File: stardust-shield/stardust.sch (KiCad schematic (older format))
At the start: 56 parts, among them J1 BEXUS 28V, J2 Pololu J8557, J3 Pololu J8557, J4 Pololu J9251, J5 Pololu J9251 Servo, J6 DS3231M, J7 VMA430, J7'1 VMA430, SW1 SW_Push, SW2 SW_Push, U1 INA181, U2 INA181, U3 INA181, U4 INA181, U5 DS18B20, U6 DS18B20, U8 DHT22, U9 SSCDRNN015PASA5

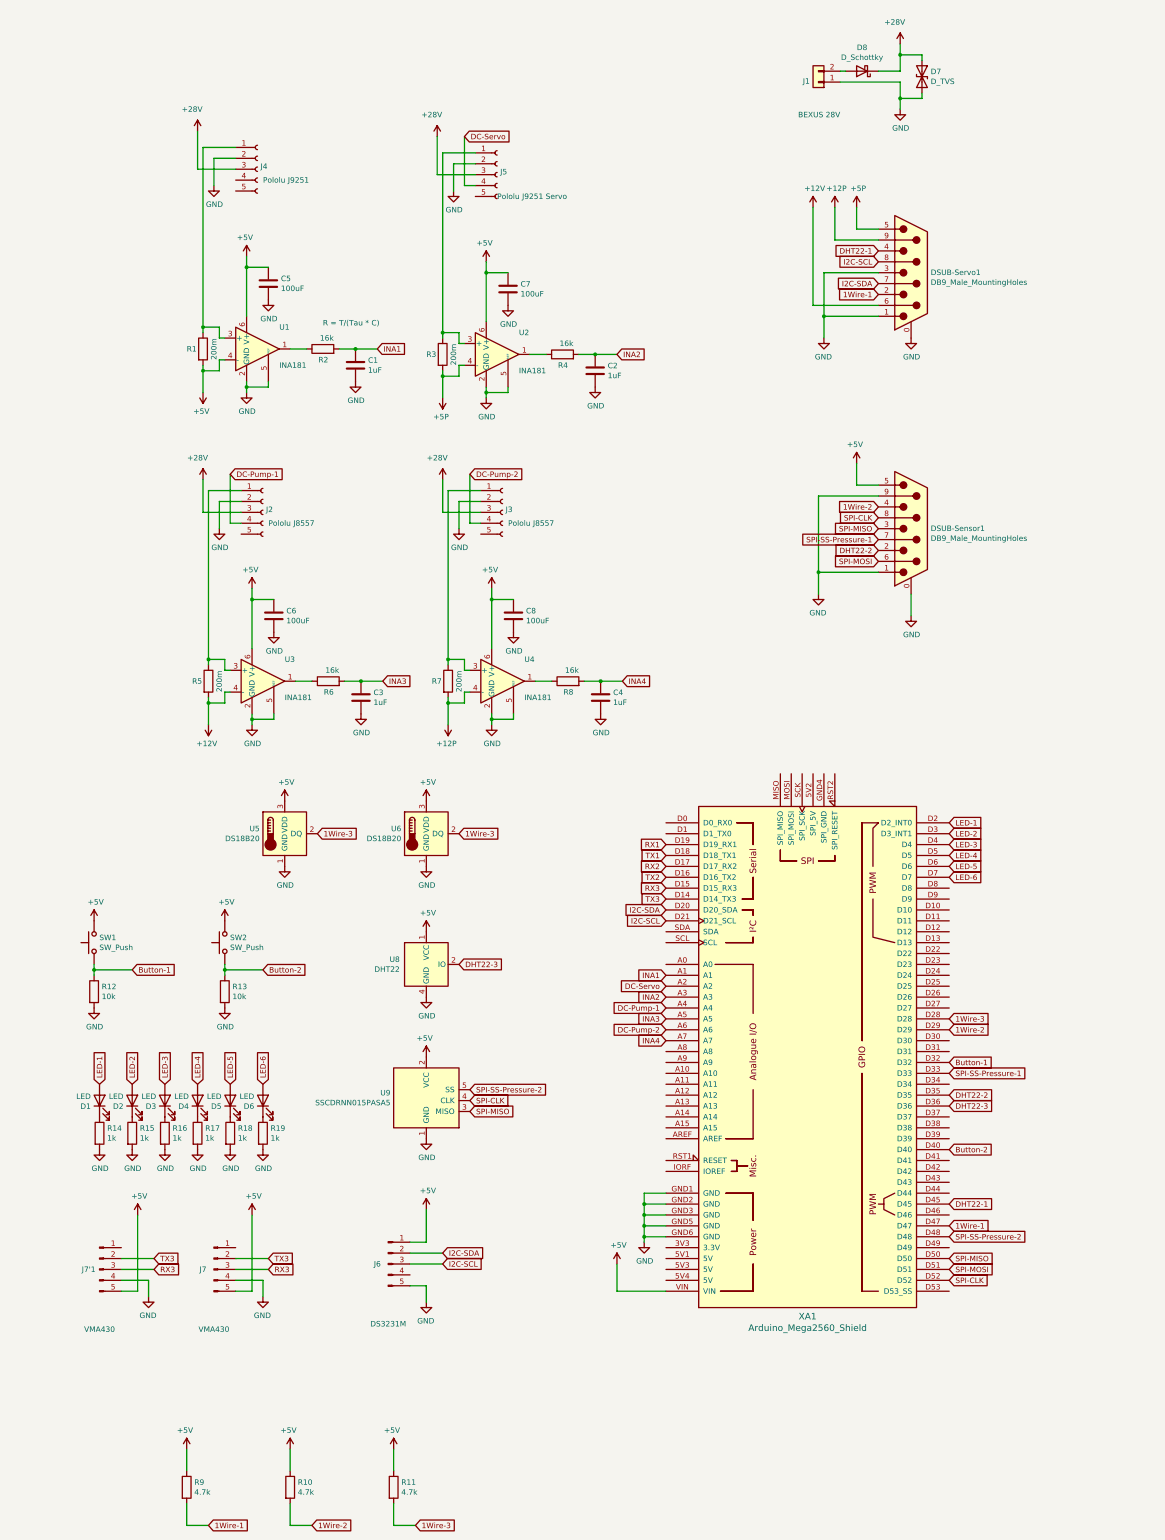
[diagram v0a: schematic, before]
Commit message: change everything
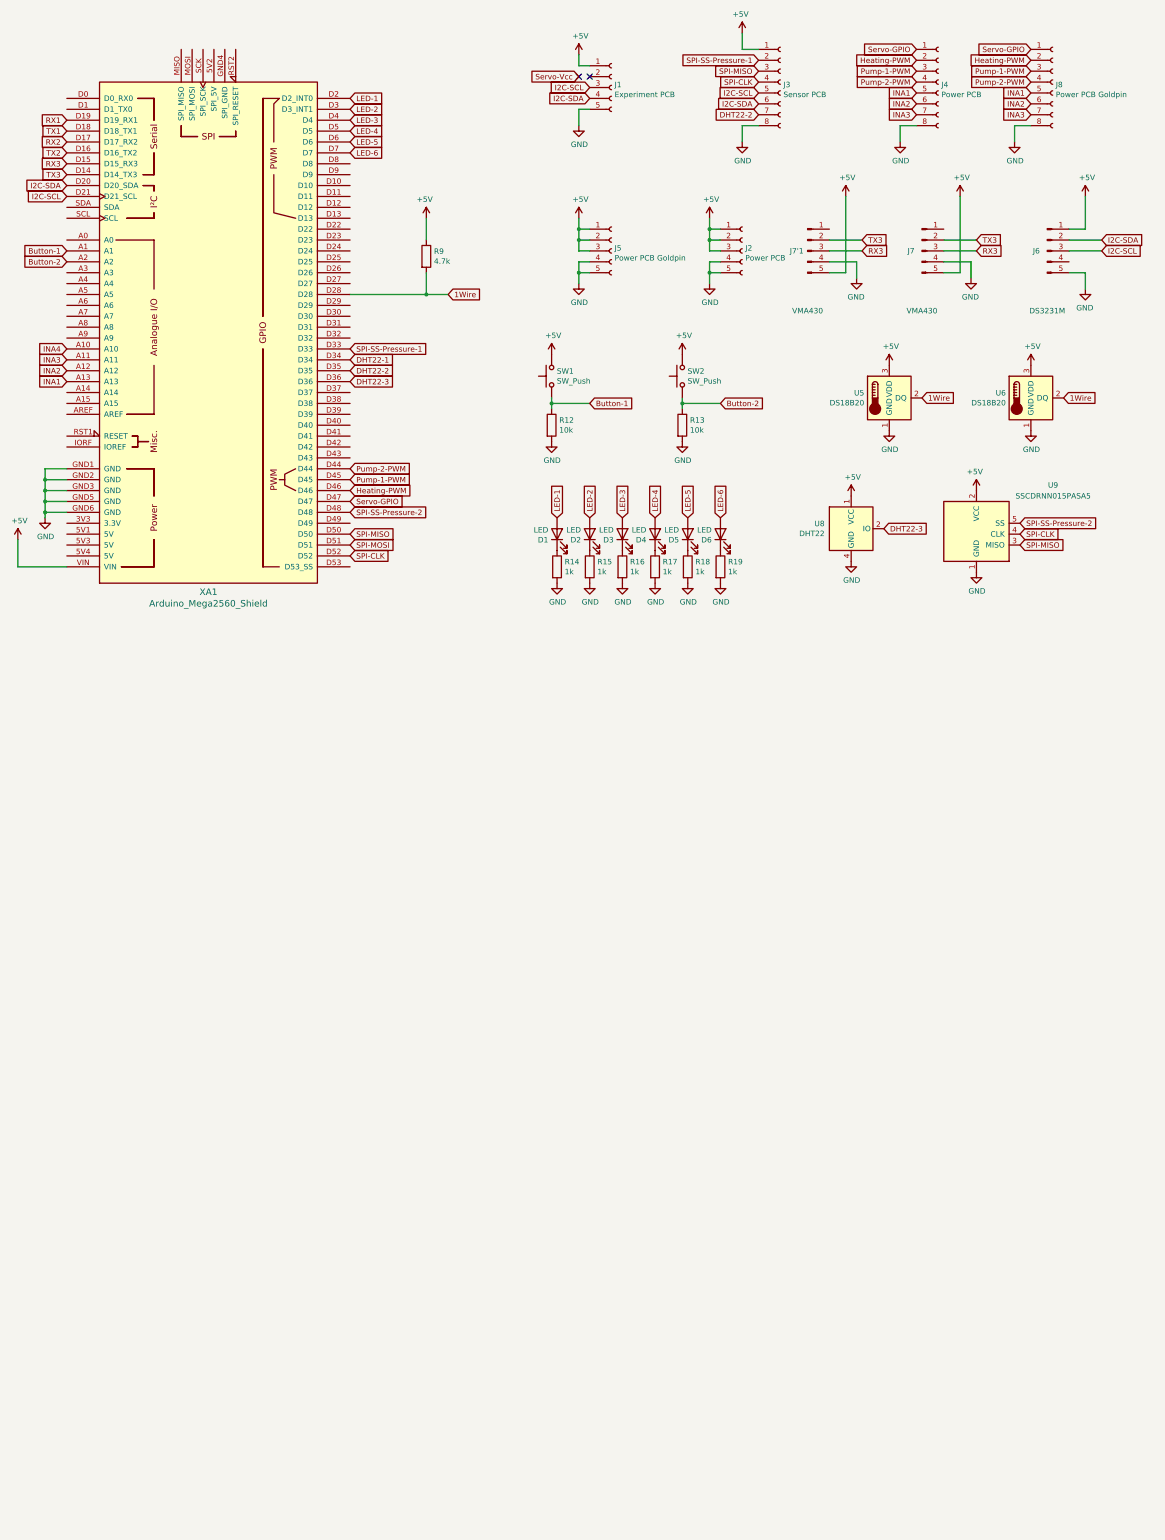
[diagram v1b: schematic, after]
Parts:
- removed C1, C2, C3, C4: 1uF, Capacitor_SMD:C_0603_1608Metric_Pad1.05x0.95mm_HandSolder, symbol Device:C
- removed C5, C6, C7, C8: 100uF, Capacitor_SMD:C_0603_1608Metric_Pad1.05x0.95mm_HandSolder, symbol Device:C
- removed D7: D_TVS, Diode_SMD:D_SMB_Handsoldering, symbol Device:D_TVS
- removed D8: D_Schottky, Diode_SMD:D_SMA, symbol Device:D_Schottky
- removed DSUB-Sensor1, DSUB-Servo1: DB9_Male_MountingHoles, Connector_Dsub:DSUB-9_Male_Horizontal_P2.77x2.84mm_EdgePinOffset7.70mm_Housed_MountingHolesOffset9.12mm, symbol stardust-rescue:DB9_Male_MountingHoles-Connector
- removed J1: BEXUS 28V, Connector_Wire:SolderWirePad_1x02_P3.81mm_Drill1.2mm, symbol stardust-rescue:Conn_01x02-Connector_Generic
- removed J2, J3: Pololu J8557, Connector_PinSocket_2.54mm:PinSocket_1x05_P2.54mm_Vertical, symbol stardust-rescue:Conn_01x05_Female-Connector
- removed J4: Pololu J9251, Connector_PinSocket_2.54mm:PinSocket_1x05_P2.54mm_Vertical, symbol stardust-rescue:Conn_01x05_Female-Connector
- removed J5: Pololu J9251 Servo, Connector_PinSocket_2.54mm:PinSocket_1x05_P2.54mm_Vertical, symbol stardust-rescue:Conn_01x05_Female-Connector
- removed R1, R3, R5, R7: 200m, Resistor_SMD:R_0603_1608Metric_Pad1.05x0.95mm_HandSolder, symbol Device:R
- removed R10, R11: 4.7k, Resistor_SMD:R_0603_1608Metric_Pad1.05x0.95mm_HandSolder, symbol Device:R
- removed R2, R4, R6, R8: 16k, Resistor_SMD:R_0603_1608Metric_Pad1.05x0.95mm_HandSolder, symbol Device:R
- removed U1, U2, U3, U4: INA181, Package_TO_SOT_SMD:SOT-23-6, symbol Amplifier_Current:INA181
- added J1: Experiment PCB, Stardust:691382000005, symbol Connector:Conn_01x05_Female
- added J2: Power PCB, Stardust:691382000005, symbol Connector:Conn_01x05_Female
- added J3: Sensor PCB, Stardust:691382030008, symbol Connector:Conn_01x08_Female
- added J4: Power PCB, Stardust:691382030008, symbol Connector:Conn_01x08_Female
- added J5: Power PCB Goldpin, Connector_PinHeader_2.54mm:PinHeader_1x05_P2.54mm_Vertical, symbol Connector:Conn_01x05_Female
- added J8: Power PCB Goldpin, Connector_PinHeader_2.54mm:PinHeader_1x08_P2.54mm_Vertical, symbol Connector:Conn_01x08_Female
- R12, R13, R14, R15, R16, R17, R18, R19, R9: footprint Resistor_SMD:R_0603_1608Metric_Pad1.05x0.95mm_HandSolder -> Resistor_SMD:R_0603_1608Metric_Pad0.98x0.95mm_HandSolder
- SW1, SW2: footprint Button_Switch_THT:SW_TH_Tactile_Omron_B3F-10xx -> Button_Switch_THT:SW_PUSH_6mm
- U8: footprint Sensor:Aosong_DHT11_5.5x12.0_P2.54mm -> Stardust:DHT22_15.0x25.0_P2.54mm_Horizontal
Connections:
- net 1Wire-3 is gone; now on net 1Wire: U5.2 (DQ), U6.2 (DQ), XA1.D28
- net DC-Servo is gone; now on net Button-2: XA1.A2
- net +5V: now also J1.1 (Pin_1), J2.1 (Pin_1), J2.2 (Pin_2), J2.3 (Pin_3), J3.1 (Pin_1), J5.1 (Pin_1), J5.2 (Pin_2), J5.3 (Pin_3)
- net Button-1: now also XA1.A1; no longer XA1.D32
- net Button-2: no longer XA1.D40
- net DHT22-1: now also XA1.D34; no longer XA1.D45
- net DHT22-2: now also J3.7 (Pin_7)
- net GND: now also J1.5 (Pin_5), J2.4 (Pin_4), J2.5 (Pin_5), J3.8 (Pin_8), J4.8 (Pin_8), J5.4 (Pin_4), J5.5 (Pin_5), J8.8 (Pin_8)
- net I2C-SCL: now also J1.3 (Pin_3), J3.5 (Pin_5)
- net I2C-SDA: now also J1.4 (Pin_4), J3.6 (Pin_6)
- net INA1: now also XA1.A13, J4.5 (Pin_5), J8.5 (Pin_5); no longer XA1.A1
- net INA2: now also XA1.A12, J4.6 (Pin_6), J8.6 (Pin_6); no longer XA1.A3
- net INA3: now also XA1.A11, J4.7 (Pin_7), J8.7 (Pin_7); no longer XA1.A5
- net INA4: now also XA1.A10; no longer XA1.A7
- net SPI-CLK: now also J3.4 (Pin_4)
- net SPI-MISO: now also J3.3 (Pin_3)
- net SPI-SS-Pressure-1: now also J3.2 (Pin_2)
- net Pump-2-PWM: now reaches XA1.D44
- net Pump-2-PWM: now also J4.4 (Pin_4), J8.4 (Pin_4)
- net Heating-PWM: now reaches XA1.D46
- net Heating-PWM: now also J4.2 (Pin_2), J8.2 (Pin_2)
- net 1Wire-1 renamed 1Wire
- net 1Wire: no longer XA1.D47
- net 1Wire-2: no longer names the net of XA1.D29
- net DC-Pump-1: no longer names the net of XA1.A4
- net DC-Pump-2: no longer names the net of XA1.A6
- new net Pump-1-PWM: J4.3 (Pin_3), J8.3 (Pin_3), XA1.D45
- new net Servo-GPIO: J4.1 (Pin_1), J8.1 (Pin_1), XA1.D47
- no-connect marks 0 -> 2
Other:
- note removed: "R = T/(Tau * C) \n"
- moved on the sheet: D1, D2, D3, D4, D5, D6, J6, J7, J7'1, R12, R13, R14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
